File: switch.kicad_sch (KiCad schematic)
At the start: 6 parts, among them Q2 2N7002, U9 74HC4052

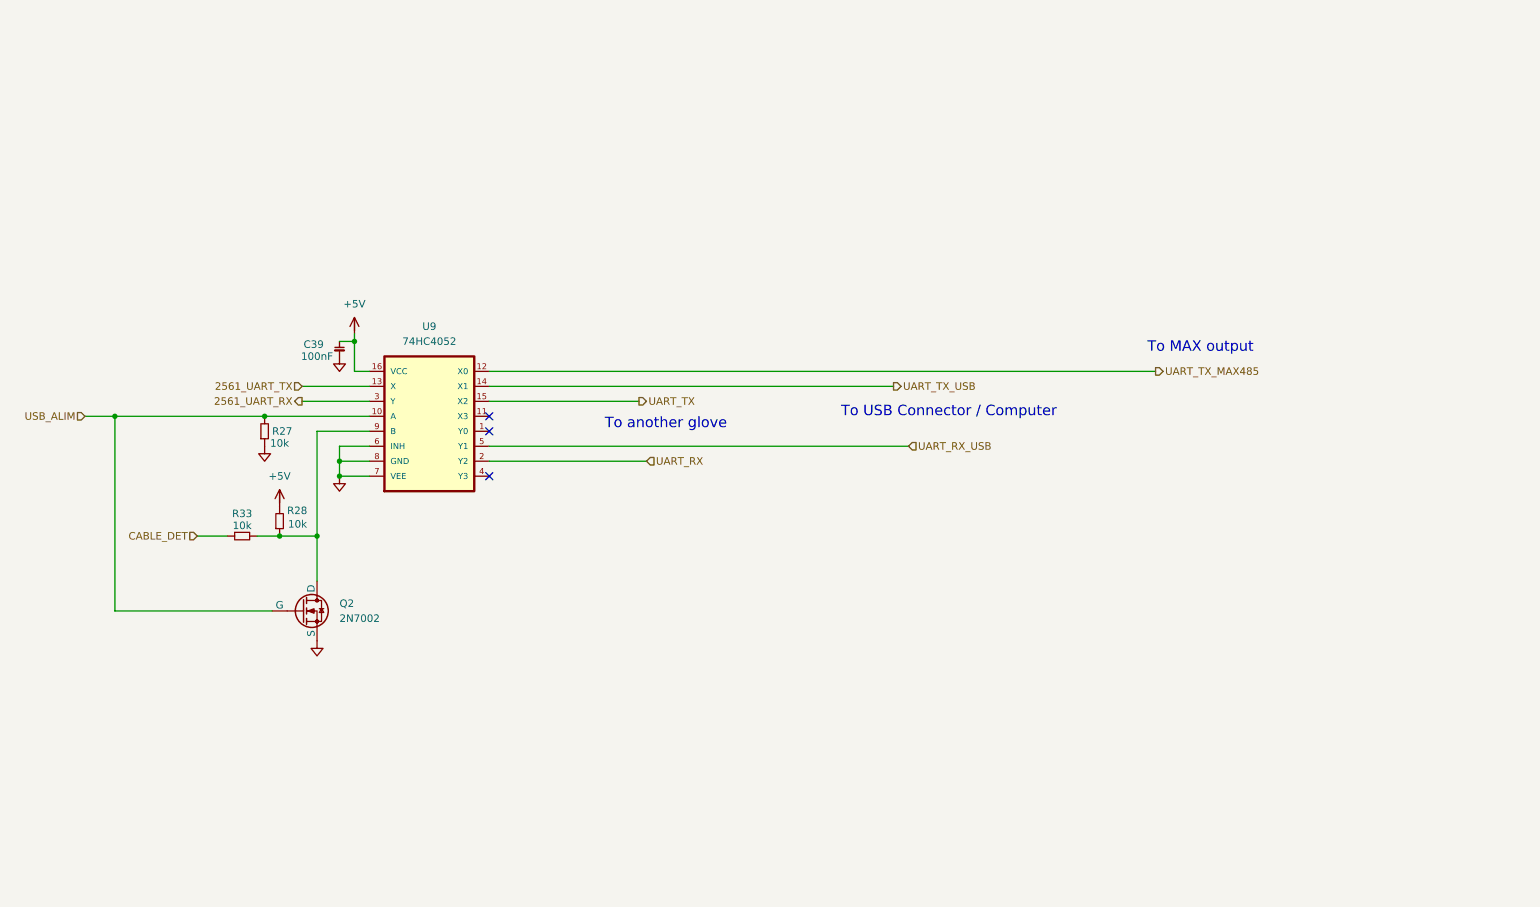
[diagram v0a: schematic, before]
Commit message: version final V1
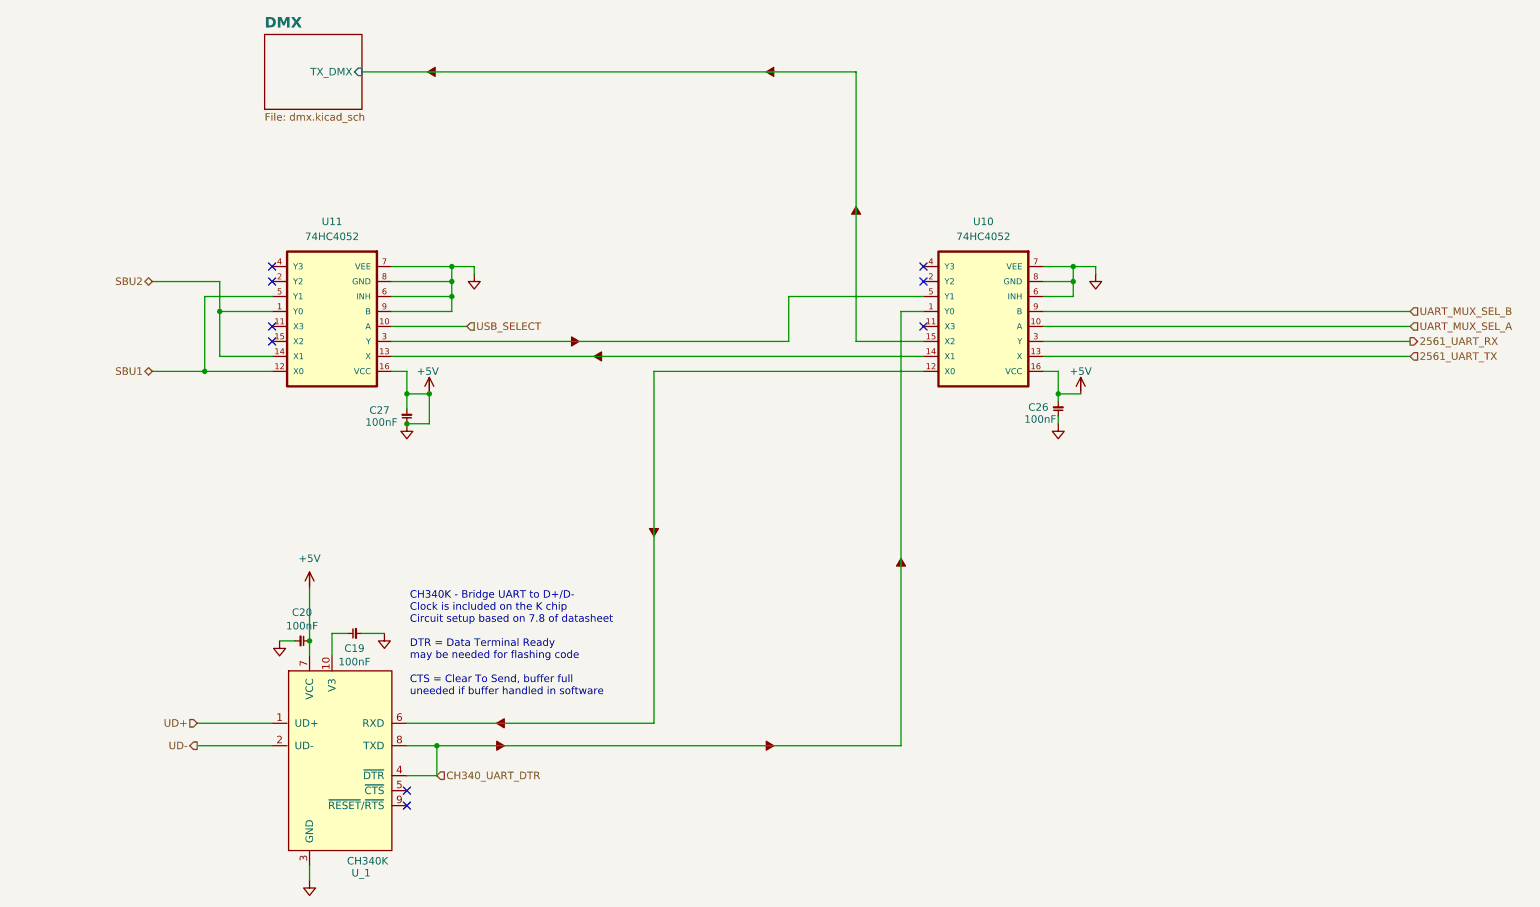
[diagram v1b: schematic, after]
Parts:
- removed C39: 100nF, symbol G-Love:C
- removed Q2: 2N7002, Package_TO_SOT_SMD:SOT-23, symbol Transistor_FET:2N7002
- removed R27, R28, R33: 10k, symbol G-Love:R
- removed U9: 74HC4052, symbol G-Love:74HC4052
- added C19, C20, C26, C27: 100nF, symbol G-Love:C
- added U10, U11: 74HC4052, symbol G-Love:74HC4052
- added U_1: CH340K, symbol G-Love:CH340K
- added flow10, flow11, flow12, flow13, flow14, flow15, flow16, flow33, flow34, flow9: (no value), symbol G-Love:FlowDirection
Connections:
- net +5V: now also C19.1, C20.1, C20.2, C26.1, C26.2, C27.1, C27.2, U10.16 (VCC), U10.6 (INH), U10.7 (VEE), U10.8 (GND), U11.16 (VCC), U11.6 (INH), U11.7 (VEE), U11.8 (GND), U11.9 (B), U_1.0 (GND), U_1.3 (GND), U_1.7 (VCC)
- net 2561_UART_RX: now also U10.3 (Y)
- net 2561_UART_TX: now also U10.13 (X)
- new net: C19.2, U_1.10 (V3)
- new net: U10.12 (X0), U_1.6 (RXD)
- new net: U10.14 (X1), U11.13 (X)
- new net: U10.5 (Y1), U11.3 (Y)
- new net CH340_UART_DTR: U10.1 (Y0), U_1.4 (~{DTR}), U_1.8 (TXD)
- new net DMX/TX_DMX: U10.15 (X2)
- new net SBU1: U11.12 (X0), U11.5 (Y1)
- new net SBU2: U11.1 (Y0), U11.14 (X1)
- new net UART_MUX_SEL_A: U10.10 (A)
- new net UART_MUX_SEL_B: U10.9 (B)
- new net UD+: U_1.1 (UD+)
- new net UD-: U_1.2 (UD-)
- new net USB_SELECT: U11.10 (A)
- no-connect marks 3 -> 9
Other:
- added sheet DMX (dmx.kicad_sch)
- note added: "CH340K - Bridge UART to D+/D- Clock is included on the K chip Circuit setup based on 7.8 of datasheet DTR = Data Terminal Ready may be needed for flashing code CTS = Clear To Send, buffer full uneeded if buffer handled in software"
- note removed: "To MAX output"
- note removed: "To USB Connector / Computer"
- note removed: "To another glove"

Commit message: add: bom
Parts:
- C19, C20, C26, C27: Price (none) -> 1.44/100; SUPPLIER (none) -> https://www.lcsc.com/product-detail/C1591.html
- U10, U11: Price None -> 0.73; SUPPLIER (none) -> https://www.lcsc.com/product-detail/C11350.html
- U_1: Price (none) -> 0.6; SUPPLIER (none) -> https://www.lcsc.com/product-detail/C968586.html
